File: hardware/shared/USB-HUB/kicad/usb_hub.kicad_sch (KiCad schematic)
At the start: 0 parts

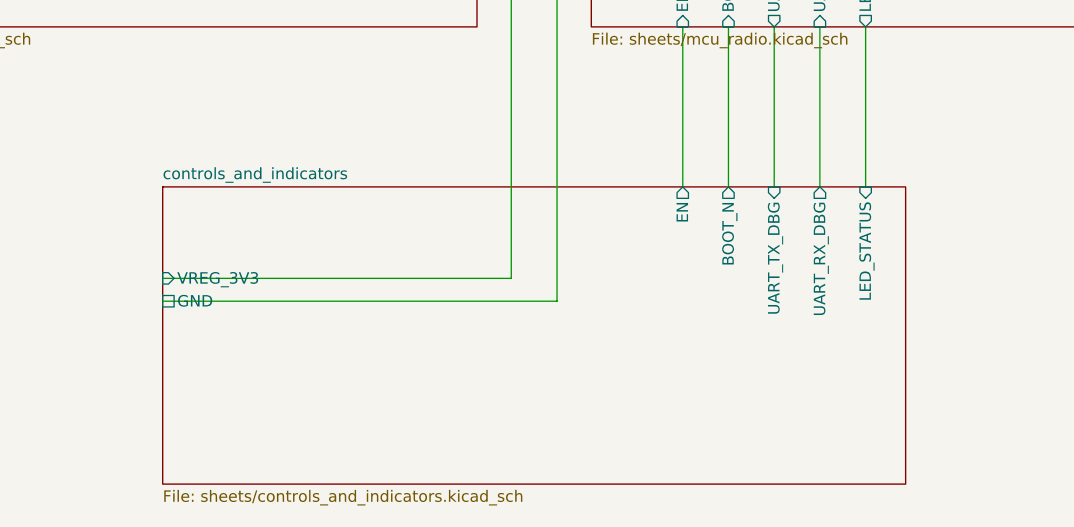
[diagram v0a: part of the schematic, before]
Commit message: fix(usb-hub): close kicad erc snapshot
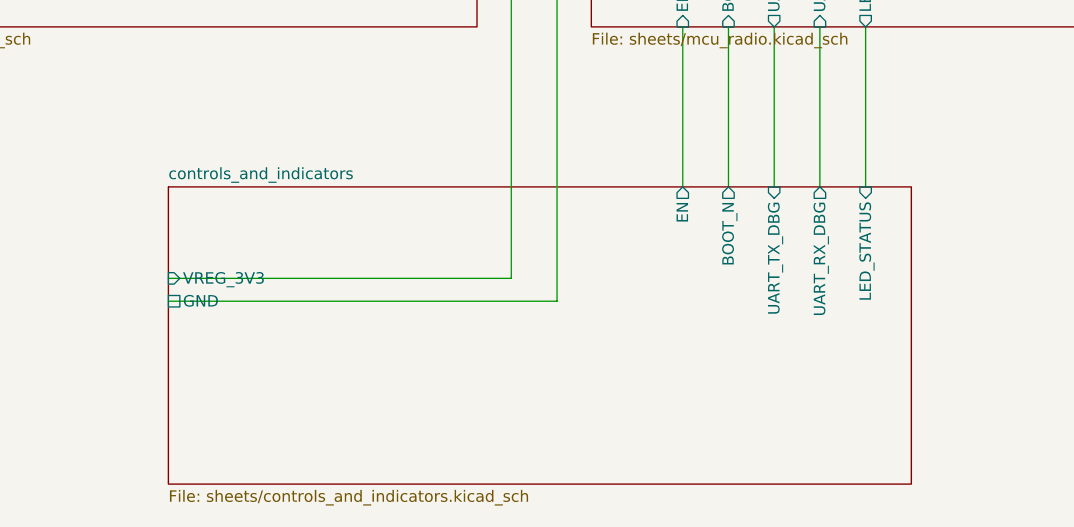
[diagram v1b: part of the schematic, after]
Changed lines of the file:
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@@
   )
   (sheet
-    (at 73.025 76.2)
+    (at 73.66 76.2)
     (size 82.55 33.02)
     (stroke (width 0.1524) (type solid) (color 0 0 0 0))
     (fill (color 0 0 0 0.0000))
-    (property "Sheet name" "controls_and_indicators" (id 0) (at 73.025 75.4884 0)
+    (property "Sheet name" "controls_and_indicators" (id 0) (at 73.66 75.4884 0)
       (effects (font (size 1.27 1.27)) (justify left bottom))
     )
-    (property "Sheet file" "sheets/controls_and_indicators.kicad_sch" (id 1) (at 73.025 109.8546 0)
+    (property "Sheet file" "sheets/controls_and_indicators.kicad_sch" (id 1) (at 73.66 109.8546 0)
       (effects (font (size 1.27 1.27)) (justify left top))
     )
@@
       (effects (font (size 1.27 1.27)))
     )
-    (pin "VREG_3V3" input (at 73.025 86.36 180)
+    (pin "VREG_3V3" input (at 73.66 86.36 180)
       (effects (font (size 1.27 1.27)) (justify left))
     )
-    (pin "GND" passive (at 73.025 88.9 180)
+    (pin "GND" passive (at 73.66 88.9 180)
       (effects (font (size 1.27 1.27)) (justify left))
     )
@@
     (pts
       (xy 111.76 86.36)
-      (xy 73.025 86.36)
+      (xy 73.66 86.36)
     )
     (stroke (width 0) (type default) (color 0 0 0 0))
@@
     (pts
       (xy 116.84 88.9)
-      (xy 73.025 88.9)
+      (xy 73.66 88.9)
     )
     (stroke (width 0) (type default) (color 0 0 0 0))
